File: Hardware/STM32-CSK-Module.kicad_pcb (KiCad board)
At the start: 2 copper layers, 54.6 x 91.4 mm, 32 parts, among them J1 Conn_Cortex-JTAG-10, U1 STM32F417VGT, X1 8MHz, X2 32.768kHz

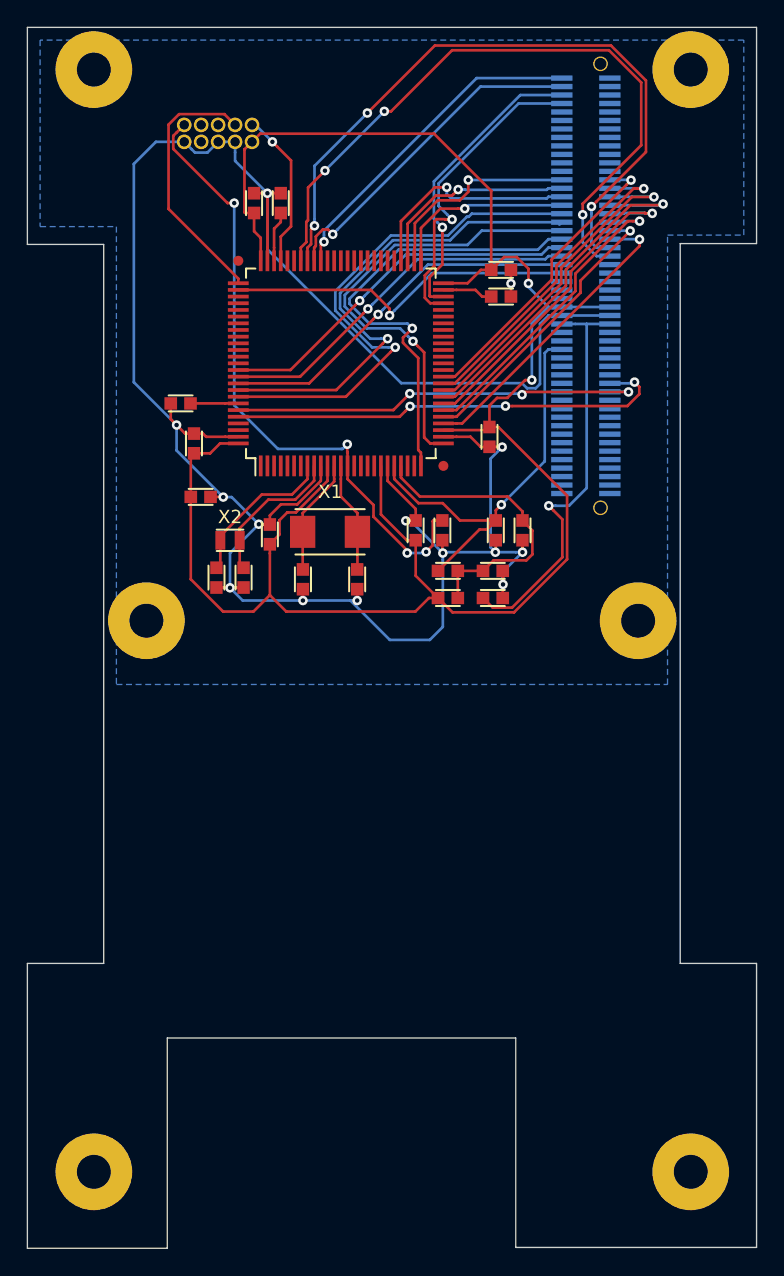
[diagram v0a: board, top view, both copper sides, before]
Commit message: Done routing it properly
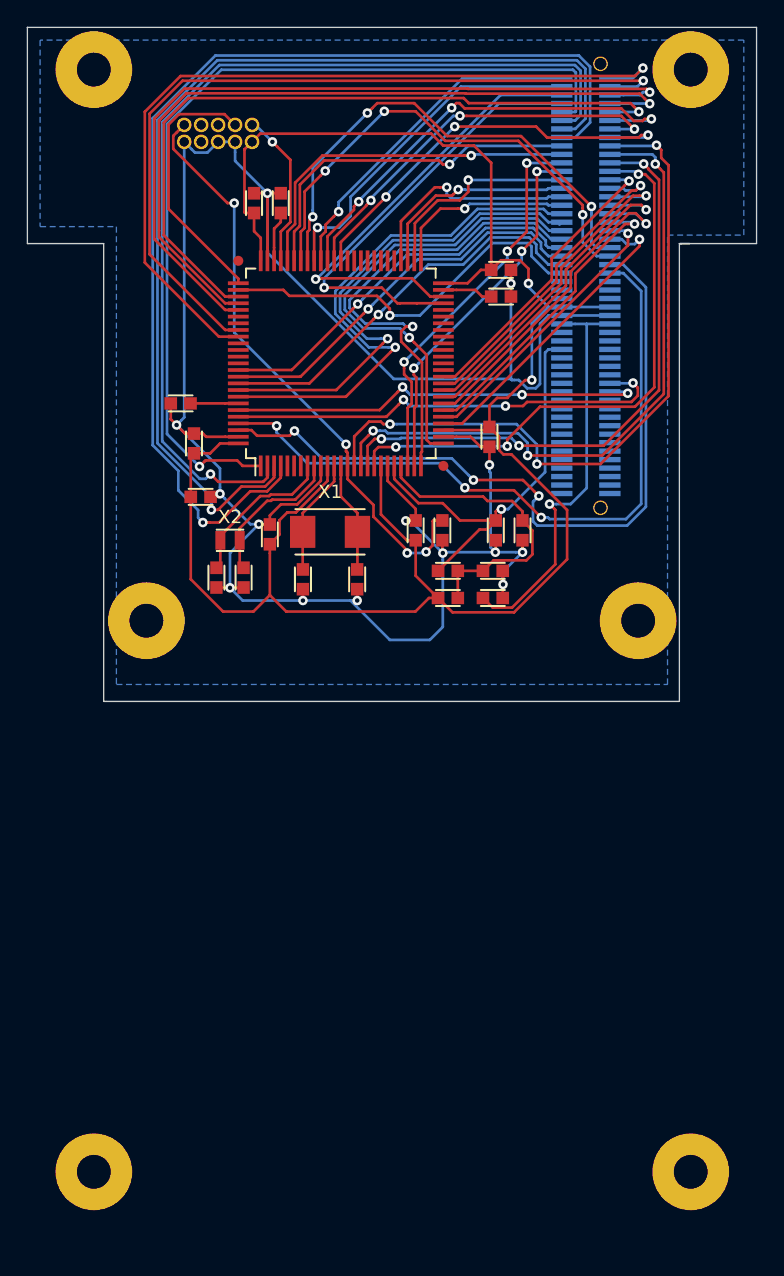
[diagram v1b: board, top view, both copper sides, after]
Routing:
- net /IO16: track 0.00 -> 81.8 mm, vias 0 -> 1
- net /IO17: track 0.00 -> 77.4 mm, vias 0 -> 1
- net /IO18: track 0.00 -> 72.5 mm, vias 0 -> 1
- net /IO19: track 0.00 -> 68.0 mm, vias 0 -> 1
- net /IO47: track 0.60 -> 62.6 mm, vias 0 -> 1
- net /IO46: track 0.00 -> 60.2 mm, vias 0 -> 1
- net /IO45: track 0.00 -> 58.7 mm, vias 0 -> 1
- net /IO44: track 0.00 -> 57.6 mm, vias 0 -> 1
- net /IO25: track 0.00 -> 56.0 mm, vias 0 -> 3
- net /IO43: track 0.00 -> 54.9 mm, vias 0 -> 1
- net /AN2: track 0.00 -> 53.2 mm, vias 0 -> 3
- net /IO24: track 0.00 -> 52.8 mm, vias 0 -> 3
- net /AN3: track 0.00 -> 49.5 mm, vias 0 -> 3
- net /AN4: track 0.00 -> 45.5 mm, vias 0 -> 3
- net /AN5: track 0.00 -> 43.3 mm, vias 0 -> 3
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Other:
- board size 54.6 x 91.4 mm -> 54.6 x 50.5 mm
